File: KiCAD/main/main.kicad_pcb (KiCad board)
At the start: 2 copper layers, 61.5 x 60.5 mm, 20 parts, among them IC1 DHT22, J1 Sound Sensor, J2 BuckConverter, J3 Charge Controller, J4 Battery Status, J5 Anemometer, J6 Conn_02x04_Odd_Even, SW1 SW_SPDT, SW2 BOOT, SW3 RESET, U1 4020, U2 4N25, U3 ESP32-WROOM-32

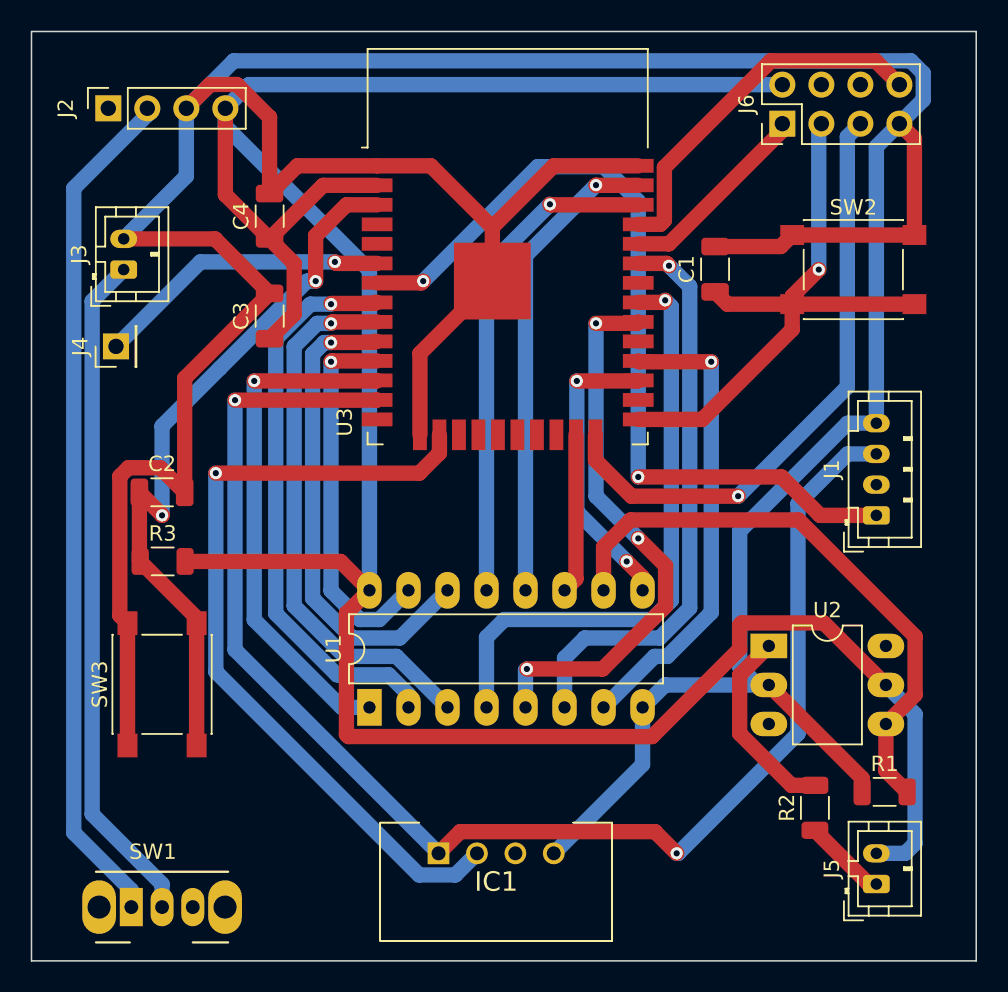
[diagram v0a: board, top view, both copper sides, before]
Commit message: Preliminary final PCB
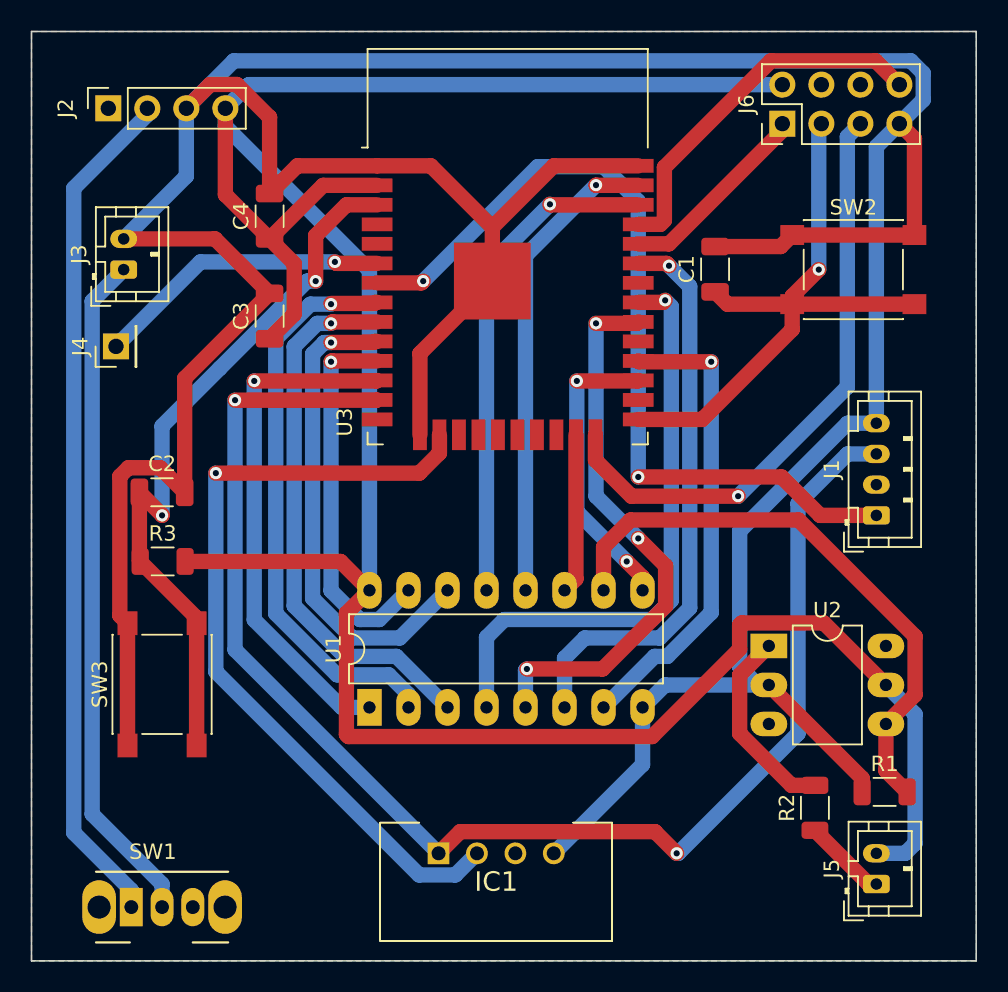
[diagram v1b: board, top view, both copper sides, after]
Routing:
- added copper zone on B.Cu, net (none)
- added copper zone on F.Cu, net (none)
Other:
- net class Default: trace_width 0.5 -> 1; via_dia 0.8 -> 1.2; via_drill 0.4 -> 0.8
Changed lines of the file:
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@@
     (zone_45_only no)
     (trace_min 0.5)
-    (via_size 0.8)
-    (via_drill 0.4)
+    (via_size 1.2)
+    (via_drill 0.8)
     (via_min_size 0.4)
     (via_min_drill 0.3)
@@
   (net_class Default "This is the default net class."
     (clearance 0.2)
-    (trace_width 0.5)
-    (via_dia 0.8)
-    (via_drill 0.4)
+    (trace_width 1)
+    (via_dia 1.2)
+    (via_drill 0.8)
     (uvia_dia 0.3)
     (uvia_drill 0.1)
@@
   (segment (start 136.445 97.635) (end 136.445 88.255) (width 1) (layer F.Cu) (net 38))
   (segment (start 135.7 98.38) (end 136.445 97.635) (width 1) (layer F.Cu) (net 38))
+  (zone (net 0) (net_name "") (layer F.Cu) (hatch edge 0.508)
+    (connect_pads (clearance 0.508))
+    (min_thickness 0.254)
+    (fill yes (arc_segments 32) (thermal_gap 0.508) (thermal_bridge_width 0.508))
+    (polygon
+      (pts
+        (xy 162.5 122.5) (xy 101 122.5) (xy 101 62) (xy 162.5 62)
+      )
+    )
+  )
+  (zone (net 0) (net_name "") (layer B.Cu) (hatch edge 0.508)
+    (connect_pads (clearance 0.508))
+    (min_thickness 0.254)
+    (fill yes (arc_segments 32) (thermal_gap 0.508) (thermal_bridge_width 0.508))
+    (polygon
+      (pts
+        (xy 162.5 122.5) (xy 101 122.5) (xy 101 62) (xy 162.5 62)
+      )
+    )
+  )
 )
